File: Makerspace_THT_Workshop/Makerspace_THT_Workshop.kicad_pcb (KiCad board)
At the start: 2 copper layers, 135.6 x 104.2 mm, 24 parts, among them SW1 SW_SPDT, U1 LM358, U2 LMC555xN

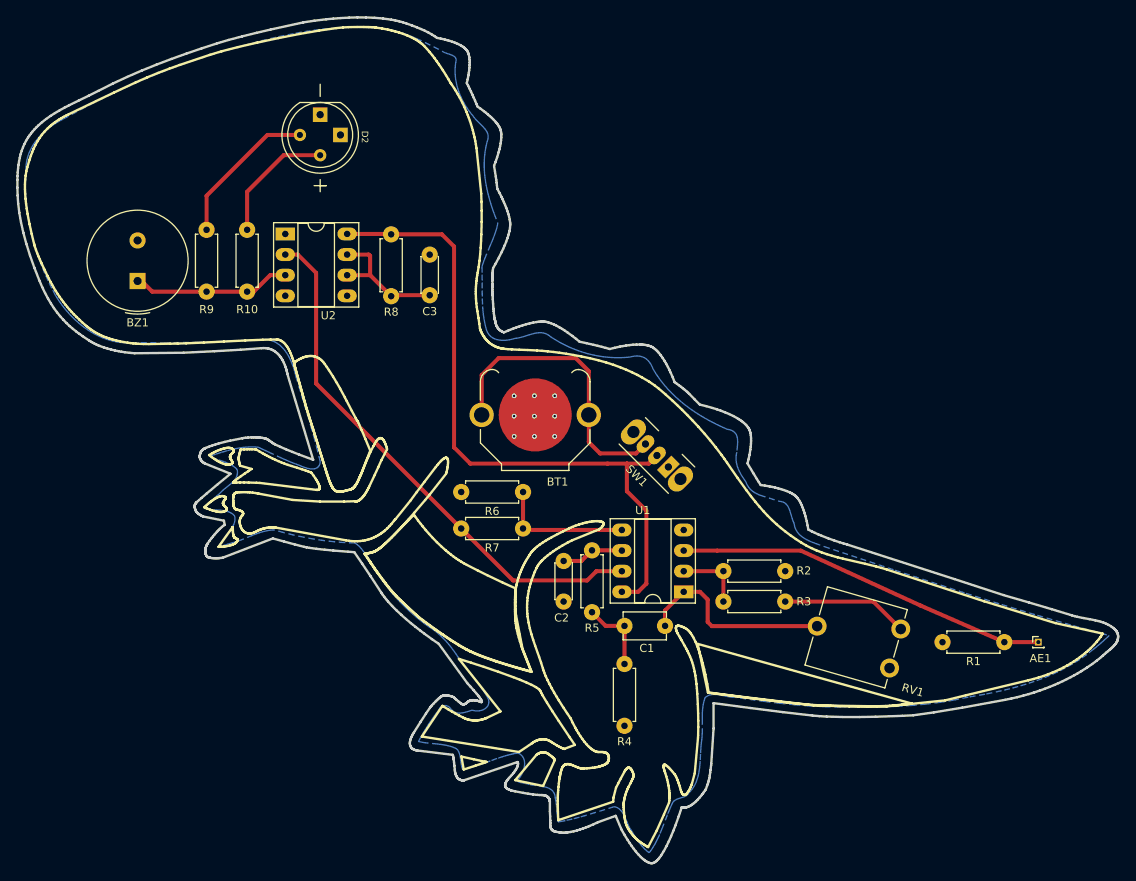
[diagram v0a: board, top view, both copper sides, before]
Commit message: Updated the board to fix alot of stuff
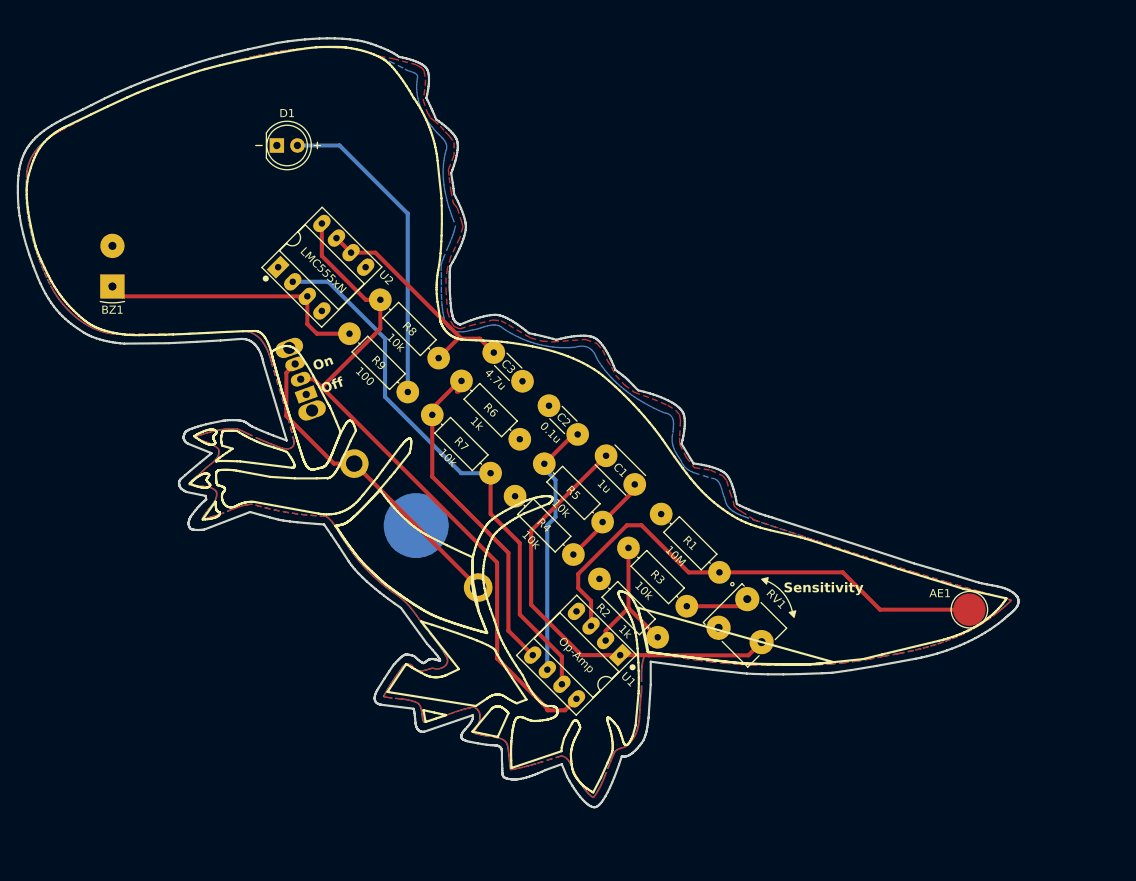
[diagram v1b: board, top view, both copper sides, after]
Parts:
- removed D2: LED, LED_THT:LED_D5.0mm_5.0mm_Pitch
- removed the G*** at (131.8, 113.5)
- removed the G*** at (147.6, 132.4)
- removed R10: 100, Resistor_THT:R_Axial_DIN0207_L6.3mm_D2.5mm_P7.62mm_Horizontal
- added G***: LOGO, Makerspace_Decals:Makerspace_Logo_20_MASKmm, B.Cu at (100.0, 75.9)
- added G***: LOGO, Makerspace_Decals:Makerspace, B.Cu at (106.2, 69.2)
- AE1: footprint Connector_PinHeader_1.00mm:PinHeader_1x01_P1.00mm_Vertical -> TestPoint:TestPoint_Pad_D4.0mm
- BT1: footprint Battery:BatteryHolder_Keystone_3001_1x12mm -> Custom_Batteries:BK-913_MPD; moved to B.Cu
- D1: footprint LED_THT:LED_D5.0mm_5.0mm_Pitch -> LED_THT:LED_D5.0mm; moved to F.Cu
- R1, R2, R3, R4, R5, R6, R7, R8, R9: footprint Resistor_THT:R_Axial_DIN0207_L6.3mm_D2.5mm_P7.62mm_Horizontal -> Resistor_THT:R_Axial_DIN0207_L6.3mm_D2.5mm_P10.16mm_Horizontal
- RV1: footprint Potentiometer_THT:Potentiometer_ACP_CA9-V10_Vertical -> Custom_Potentiometer:601030_AVX
- SW1: moved to B.Cu
- U1: value LM358 -> Op-Amp
- moved SW1 45.5 mm to (117.9, 96.1), turned to 110 degrees
- moved R1 36.1 mm to (168.8, 118.0), turned to 135 degrees
- moved C2 24.2 mm to (147.8, 97.5), turned to -45 degrees
- moved R2 22.9 mm to (154.0, 118.8), turned to -45 degrees
- moved C1 22.2 mm to (154.8, 103.6), turned to -45 degrees
- moved BT1 20.0 mm to (131.4, 112.2), turned to 135 degrees
- moved RV1 19.3 mm to (172.2, 121.3), turned to -135 degrees
- moved R9 18.4 mm to (123.2, 88.6), turned to -45 degrees
- moved R7 17.9 mm to (133.4, 98.6), turned to -45 degrees
- moved R6 15.6 mm to (137.0, 94.4), turned to -45 degrees
- moved R4 14.9 mm to (150.8, 115.8), turned to 135 degrees
- moved R3 13.4 mm to (157.6, 115.0), turned to -45 degrees
- moved R5 11.2 mm to (154.4, 111.8), turned to 135 degrees
- moved U1 11.0 mm to (156.6, 128.2), turned to -135 degrees
- moved C3 10.6 mm to (141.0, 90.9), turned to -45 degrees
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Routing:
- net Net-(C1-Pad1): track 25.0 -> 53.8 mm
- net Net-(U1B--): track 7.74 -> 32.0 mm
- net Net-(U1B-+): track 16.8 -> 40.7 mm
- net Net-(D1-A): track 18.8 -> 39.1 mm
- net Net-(AE1-A): track 46.1 -> 62.1 mm
- net Net-(D2-A): track 15.6 -> 0.00 mm
- net Net-(BZ1-+): track 19.6 -> 33.6 mm
- net Net-(U2-DIS): track 16.6 -> 29.0 mm
- net Net-(U1A--): track 8.66 -> 17.4 mm
- net Net-(R3-Pad2): track 15.6 -> 7.96 mm
- net Net-(BT1-+): track 36.4 -> 39.3 mm
- net Net-(C1-Pad2): track 9.39 -> 11.8 mm
- net +3V0: track 84.0 -> 85.7 mm
- net Net-(U2-TR): track 66.6 -> 68.0 mm
- net GND: vias 9 -> 0
- added copper zone on F.Cu, net GND
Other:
- board size 135.6 x 104.2 mm -> 123.3 x 94.8 mm
- board text added: "AC Dino Voltage Detector V2.0"
- board text added: "Designed By: Austin Nguyen"
- board text added: "Off"
- board text added: "On"
- board text added: "Sensitivity"
- board text removed: "*Only works on alternating sources"
- board text removed: "Designed by: Austin Nguyen"
- board text removed: "Dino Sniffer Voltage Detecting Dino V1.0"
